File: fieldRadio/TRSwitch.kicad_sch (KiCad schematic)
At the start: 36 parts, among them Q1 MMBT3904, Q2 MMBT3904, Q3 PMV240SP, Q5 MMBT3904, Q6 PMV240SP, Q7 BSS123

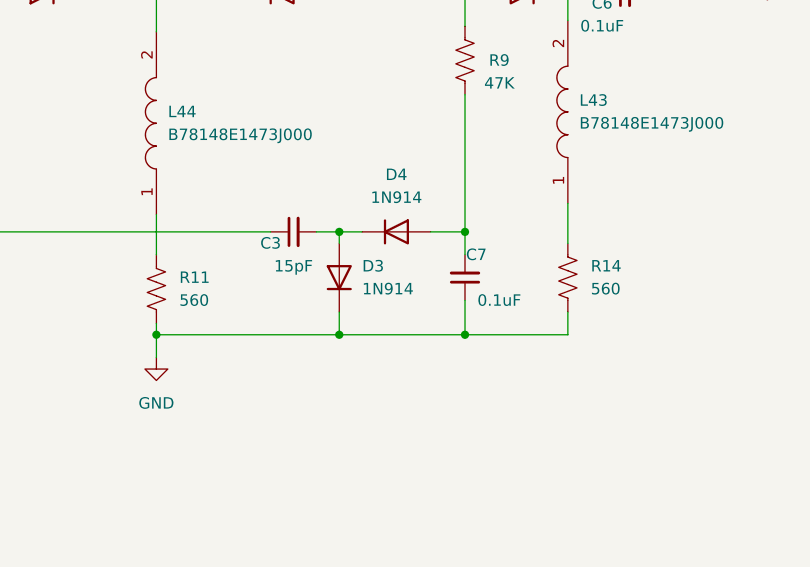
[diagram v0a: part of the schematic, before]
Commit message: First Clean DRC
first clean drc
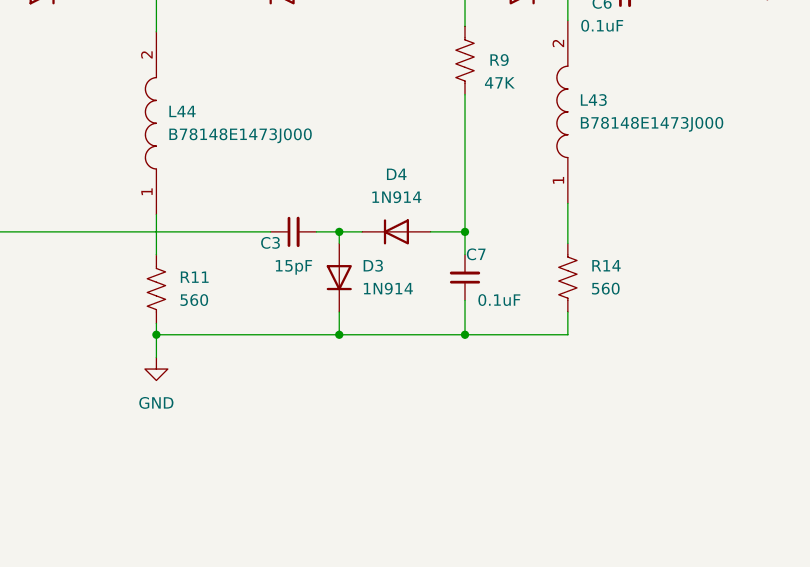
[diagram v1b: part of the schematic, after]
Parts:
- R11, R14: footprint Resistor_THT:R_Axial_DIN0411_L9.9mm_D3.6mm_P15.24mm_Horizontal -> Resistor_THT:R_Axial_DIN0617_L17.0mm_D6.0mm_P20.32mm_Horizontal
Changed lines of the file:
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@@
   (symbol (lib_id "Device:R_US") (at 265.43 147.32 0) (unit 1)
     (in_bom yes) (on_board yes) (dnp no) (fields_autoplaced)
-    (property "Reference" "R11" (at 267.97 146.0499 0)
-      (effects (font (size 1.27 1.27)) (justify left))
-    )
-    (property "Value" "560" (at 267.97 148.5899 0)
-      (effects (font (size 1.27 1.27)) (justify left))
-    )
-    (property "Footprint" "Resistor_THT:R_Axial_DIN0411_L9.9mm_D3.6mm_P15.24mm_Horizontal" (at 266.446 147.574 90)
+    (property "Reference" "R11" (at 267.97 146.05 0)
+      (effects (font (size 1.27 1.27)) (justify left))
+    )
+    (property "Value" "560" (at 267.97 148.59 0)
+      (effects (font (size 1.27 1.27)) (justify left))
+    )
+    (property "Footprint" "Resistor_THT:R_Axial_DIN0617_L17.0mm_D6.0mm_P20.32mm_Horizontal" (at 266.446 147.574 90)
       (effects (font (size 1.27 1.27)) hide)
     )
@@
   (symbol (lib_id "Device:R_US") (at 311.15 146.05 0) (unit 1)
     (in_bom yes) (on_board yes) (dnp no) (fields_autoplaced)
-    (property "Reference" "R14" (at 313.69 144.7799 0)
-      (effects (font (size 1.27 1.27)) (justify left))
-    )
-    (property "Value" "560" (at 313.69 147.3199 0)
-      (effects (font (size 1.27 1.27)) (justify left))
-    )
-    (property "Footprint" "Resistor_THT:R_Axial_DIN0411_L9.9mm_D3.6mm_P15.24mm_Horizontal" (at 312.166 146.304 90)
-      (effects (font (size 1.27 1.27)) hide)
-    )
+    (property "Reference" "R14" (at 313.69 144.78 0)
+      (effects (font (size 1.27 1.27)) (justify left))
+    )
+    (property "Value" "560" (at 313.69 147.32 0)
+      (effects (font (size 1.27 1.27)) (justify left))
+    )
+    (property "Footprint" "Resistor_THT:R_Axial_DIN0617_L17.0mm_D6.0mm_P20.32mm_Horizontal" (at 312.166 146.304 90)
+      (effects (font (size 1.27 1.27)) hide)
+    )
